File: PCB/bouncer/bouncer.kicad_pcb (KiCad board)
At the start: 2 copper layers, 70.1 x 47.1 mm, 15 parts, among them J1 Conn_01x08_Female, SW1 SW_Push_Dual, SW2 SW_Push_Dual, SW3 SW_Push_Dual, U1 74HC14

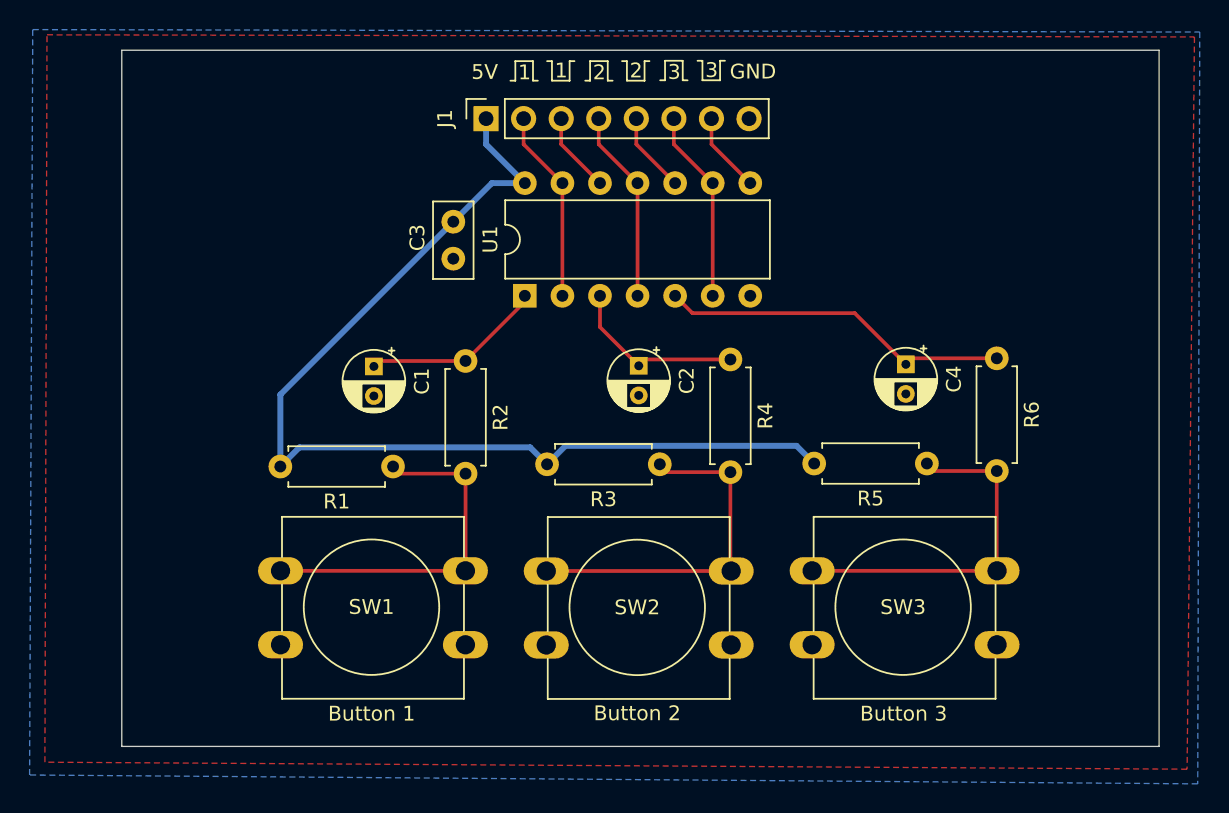
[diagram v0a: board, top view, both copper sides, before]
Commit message: rc1 for SPI Gate (prev SPI master) rc1 for Bouncer
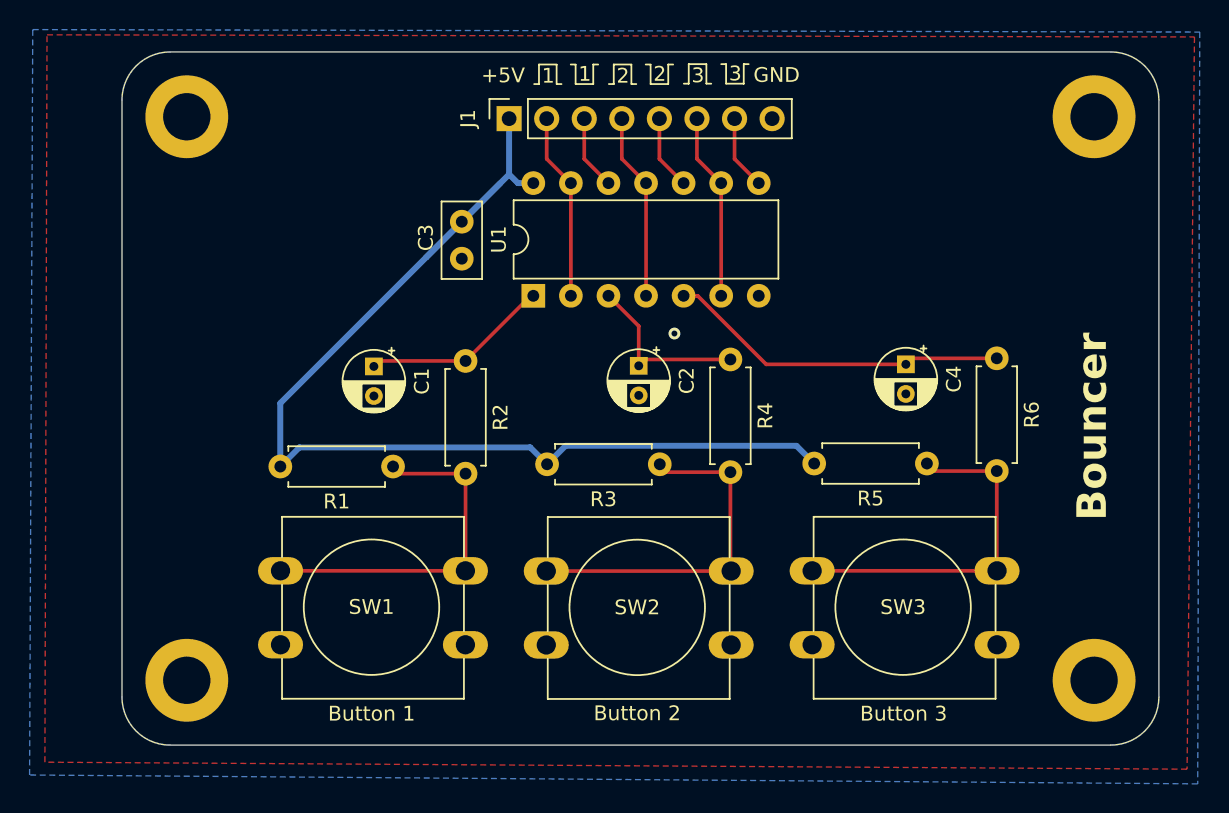
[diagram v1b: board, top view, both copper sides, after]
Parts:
- added H1: MountingHole, MountingHole:MountingHole_3.2mm_M3_DIN965_Pad, F.Cu at (129.0, 81.4)
- added H2: MountingHole, MountingHole:MountingHole_3.2mm_M3_DIN965_Pad, F.Cu at (190.4, 81.4)
- added H3: MountingHole, MountingHole:MountingHole_3.2mm_M3_DIN965_Pad, F.Cu at (129.0, 119.5)
- added H4: MountingHole, MountingHole:MountingHole_3.2mm_M3_DIN965_Pad, F.Cu at (190.4, 119.5)
- moved J1 1.56 mm to (150.8, 81.5)
- moved C3 0.57 mm to (147.6, 88.5)
- moved U1 0.57 mm to (152.5, 93.5)
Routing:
- net +5V: track 70.9 -> 77.0 mm
- net Net-(C1-Pad1): track 12.4 -> 13.2 mm
- net Net-(C4-Pad1): track 23.8 -> 23.3 mm
- net GND: vias 0 -> 1
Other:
- board size 70.1 x 47.1 mm -> 70.1 x 46.9 mm
- board text added: "+5V"
- board text added: "Bouncer"
- board text added: "v1.0 by Nate Rivard Nov 2024"
- board text removed: "5V"
